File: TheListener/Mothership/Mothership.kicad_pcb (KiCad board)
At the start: 2 copper layers, 82 x 93.5 mm, 64 parts, among them J1 RJ45, J10 Conn_01x10_Female, J11 Conn_01x10_Female, J2 RJ45, J3 RJ45, J4 RJ45, J5 RJ45, J6 RJ45, J7 RJ45, J8 RJ45, U1 SP3491, U10 AMS1117-3.3, U2 SP3491, U3 SP3491, U4 SP3491, U5 SP3491, U6 SP3491, U7 SP3491, U8 SP3491, U9 AMS1117-3.3

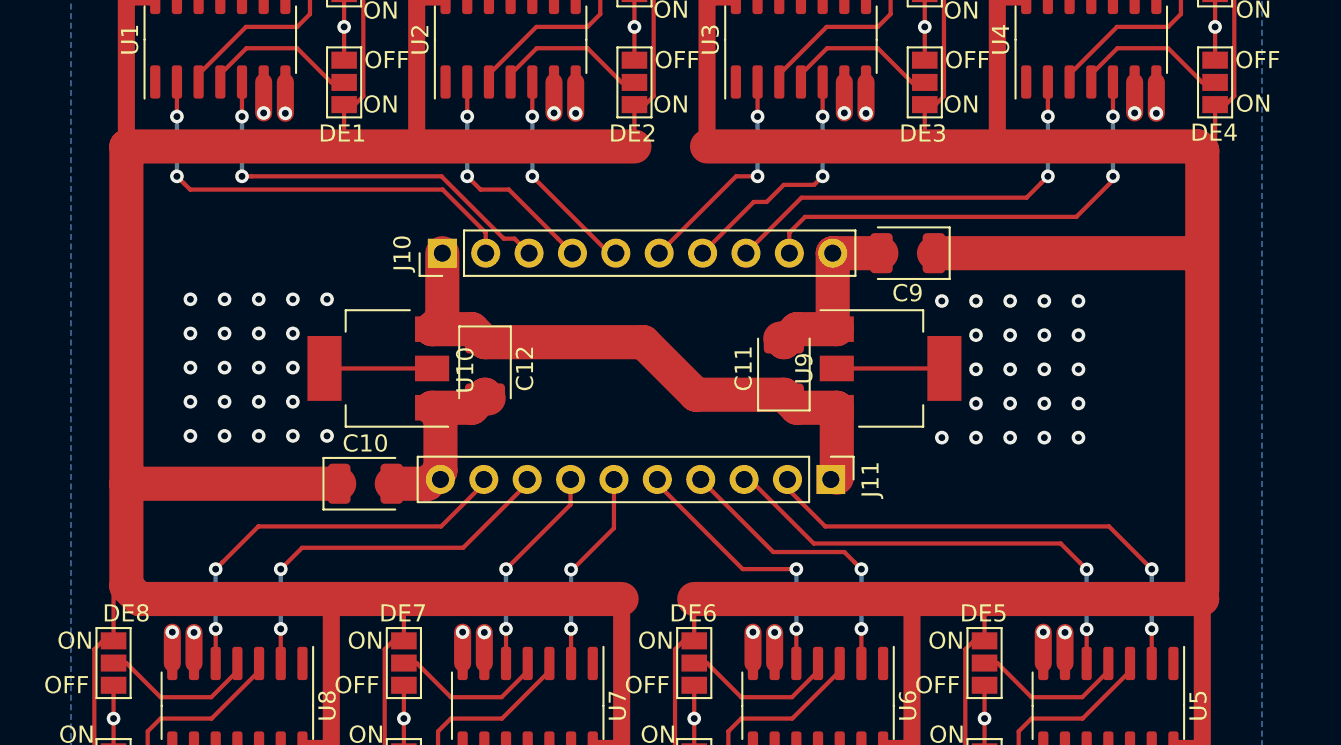
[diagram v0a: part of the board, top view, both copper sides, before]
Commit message: updates
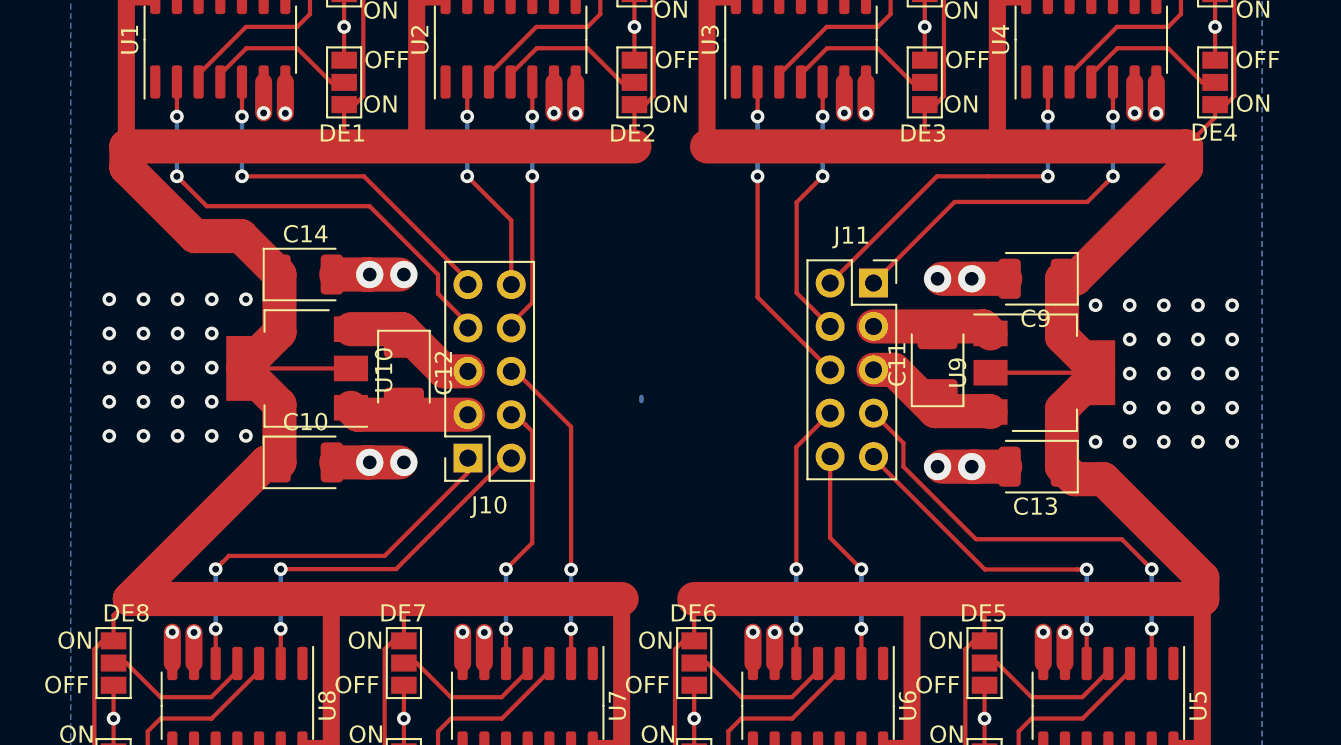
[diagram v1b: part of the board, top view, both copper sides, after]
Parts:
- added C13: 10uF, Capacitor_Tantalum_SMD:CP_EIA-3528-21_Kemet-B, F.Cu at (120.5, 73.8)
- added C14: 10uF, Capacitor_Tantalum_SMD:CP_EIA-3528-21_Kemet-B, F.Cu at (77.8, 62.5)
- C10, C9: value 22uF -> 10uF
- J10, J11: value Conn_01x10_Female -> Conn_02x05_Odd_Even; footprint Connector_PinHeader_2.54mm:PinHeader_1x10_P2.54mm_Vertical -> Connector_PinSocket_2.54mm:PinSocket_2x05_P2.54mm_Vertical
- moved J10 12.1 mm to (87.2, 73.2), turned to 180 degrees
- moved J11 11.8 mm to (111.0, 63.0), turned to 0 degrees
- moved C11 9.00 mm to (114.8, 67.8)
- moved U9 9.00 mm to (121.0, 68.2)
- moved C9 7.65 mm to (120.5, 62.8)
- moved C12 4.76 mm to (83.5, 68.2)
- moved U10 4.75 mm to (77.2, 68.0)
- moved C10 3.72 mm to (77.8, 73.5)
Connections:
- J10 pad 1: +5V -> T_5
- J10 pad 10: GND -> R_3
- J10 pad 2: R_4 -> R_5
- J10 pad 3: T_4 -> GND
- J10 pad 4: R_3 -> T_6
- J10 pad 5: T_3 -> +5V
- J10 pad 6: R_2 -> R_6
- J10 pad 7: T_2 -> R_4
- J10 pad 8: R_1 -> T_3
- J10 pad 9: T_1 -> T_4
- J11 pad 1: +5V -> T_1
- J11 pad 10: GND -> R_7
- J11 pad 2: R_8 -> R_1
- J11 pad 3: T_8 -> GND
- J11 pad 4: R_7 -> T_2
- J11 pad 5: T_7 -> +5V
- J11 pad 6: R_6 -> R_2
- J11 pad 7: T_6 -> R_8
- J11 pad 8: R_5 -> T_7
- J11 pad 9: T_5 -> T_8
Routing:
- net +5V: track 34.5 -> 15.7 mm
- net VCC1: track 205.7 -> 193.6 mm
- net GND: track 110.7 -> 118.9 mm, vias 92 -> 100
- net R_6: track 11.5 -> 18.8 mm
- net T_8: track 27.8 -> 20.7 mm
- net R_2: track 13.1 -> 18.6 mm
- net T_1: track 26.9 -> 21.5 mm
- net R_7: track 17.1 -> 12.9 mm
- net R_1: track 25.1 -> 20.9 mm
- net T_6: track 12.1 -> 16.0 mm
- net T_4: track 24.2 -> 21.3 mm
- net VCC2: track 199.4 -> 196.8 mm
- net R_8: track 28.8 -> 26.4 mm
- net T_3: track 12.3 -> 14.7 mm
- net T_2: track 14.4 -> 15.8 mm
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
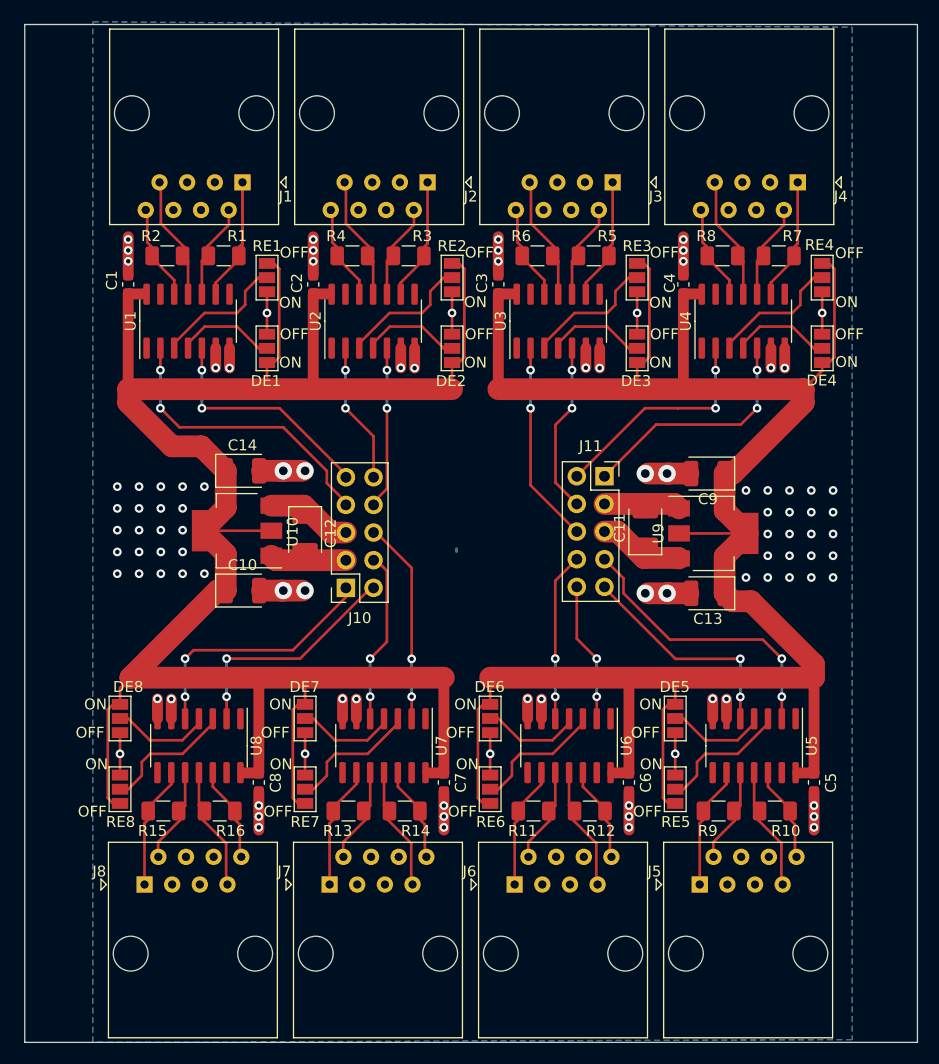
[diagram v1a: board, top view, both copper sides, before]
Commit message: final
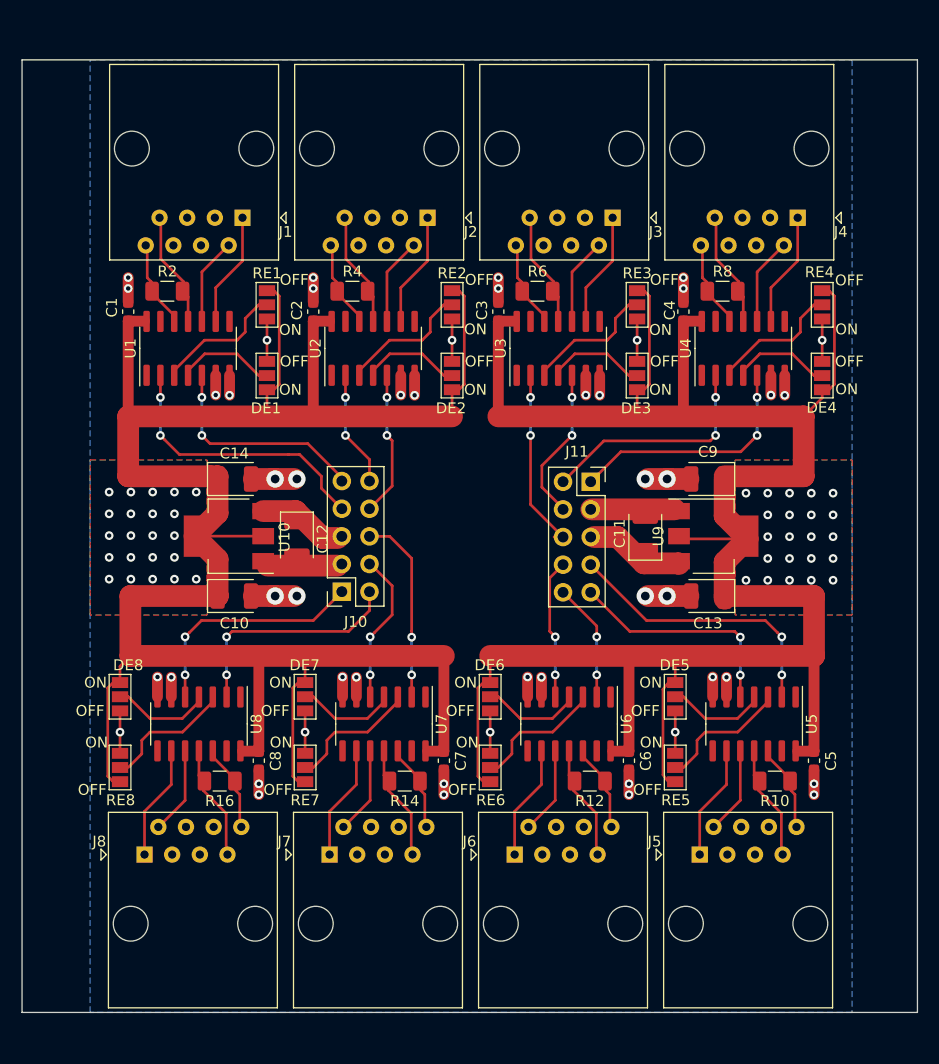
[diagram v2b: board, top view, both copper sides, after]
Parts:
- removed R1, R11, R13, R15, R3, R5, R7, R9: 100, Resistor_SMD:R_1206_3216Metric
- moved J1 3.25 mm to (77.8, 39.2)
- moved J2 3.25 mm to (94.8, 39.2)
- moved J3 3.25 mm to (111.8, 39.2)
- moved J4 3.25 mm to (128.8, 39.2)
- moved R2 3.25 mm to (70.8, 46.0)
- moved R4 3.25 mm to (87.8, 46.0)
- moved R6 3.25 mm to (104.8, 46.0)
- moved R8 3.25 mm to (121.8, 46.0)
- moved J5 2.75 mm to (119.8, 97.8)
- moved J6 2.75 mm to (102.8, 97.8)
- moved J7 2.75 mm to (85.8, 97.8)
- moved J8 2.75 mm to (68.8, 97.8)
- moved R10 2.75 mm to (126.7, 91.0)
- moved R12 2.75 mm to (109.7, 91.0)
- moved R14 2.75 mm to (92.7, 91.0)
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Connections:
- C11 pad 1: +5V -> 5VDC_1
- C12 pad 1: +5V -> 5VDC_2
- J10 pad 5: +5V -> 5VDC_2
- J11 pad 5: +5V -> 5VDC_1
- U10 pad 3: +5V -> 5VDC_2
- U9 pad 3: +5V -> 5VDC_1
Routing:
- net +5V: track 15.7 -> 0.00 mm
- net VCC2: track 196.8 -> 207.2 mm, vias 0 -> 22
- net GND: track 118.9 -> 108.7 mm, vias 100 -> 48
- net VCC1: track 193.6 -> 203.1 mm, vias 0 -> 22
- net 5VDC_1: track 0.00 -> 8.83 mm
- net 5VDC_2: track 0.00 -> 7.87 mm
- net Net-(J1-Pad1): track 17.4 -> 11.3 mm
- net T_7: track 15.5 -> 12.9 mm
- net T_5: track 23.7 -> 21.6 mm
- net T_6: track 16.0 -> 13.9 mm
- net R_3: track 12.7 -> 10.6 mm
- net R_7: track 12.9 -> 10.9 mm
- net T_2: track 15.8 -> 14.3 mm
- net R_6: track 18.8 -> 17.4 mm
- net T_3: track 14.7 -> 13.3 mm
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- added copper zone on B.Cu, net VCC1
- added copper zone on F.Cu, net VCC1
- added copper zone on B.Cu, net VCC2
- added copper zone on F.Cu, net VCC2
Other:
- board size 82 x 93.5 mm -> 82.2 x 87.5 mm

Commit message: working
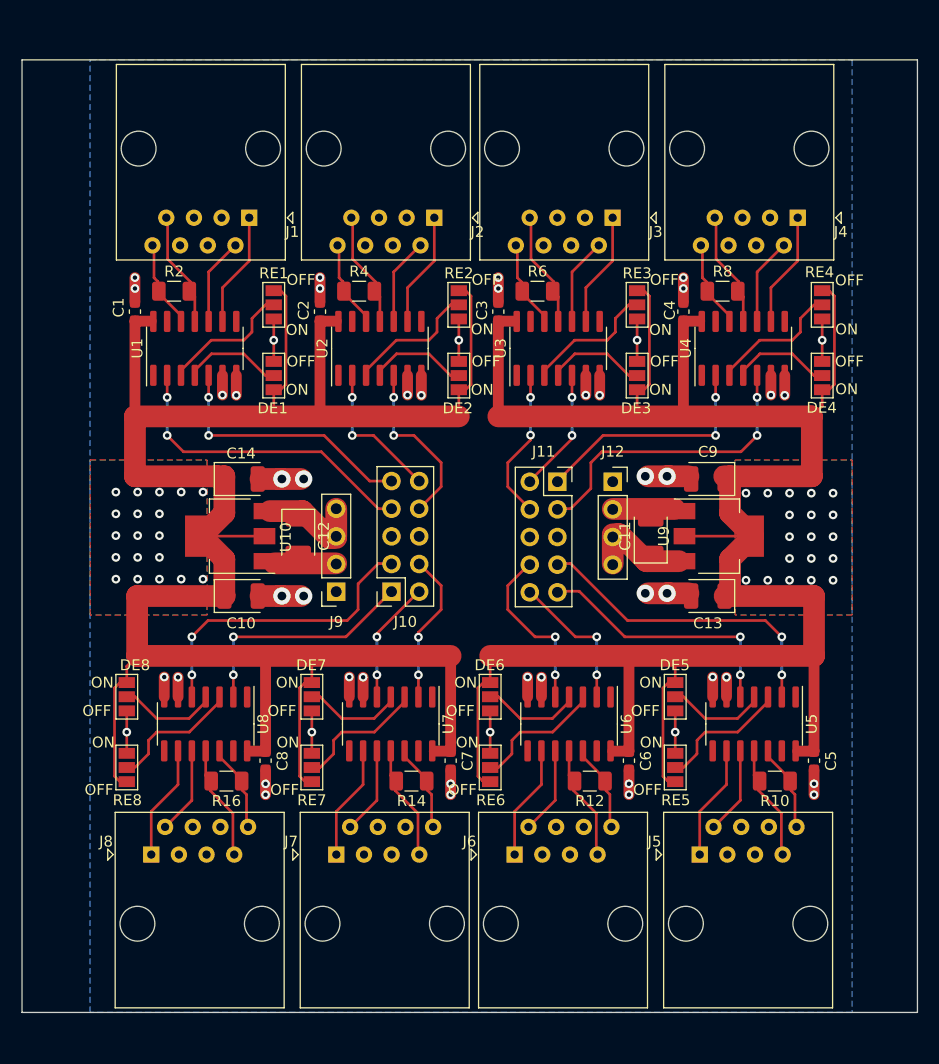
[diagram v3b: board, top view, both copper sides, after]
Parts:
- added J12: Conn_01x04_Male, Connector_PinSocket_2.54mm:PinSocket_1x04_P2.54mm_Vertical, F.Cu at (111.8, 63.5)
- added J9: Conn_01x04_Male, Connector_PinSocket_2.54mm:PinSocket_1x04_P2.54mm_Vertical, F.Cu at (86.4, 73.6)
- moved J10 4.56 mm to (91.4, 73.6)
- moved J11 3.05 mm to (106.7, 63.5)
- moved C1 0.62 mm to (67.9, 47.9)
- moved C10 0.62 mm to (77.6, 74.0)
- moved C14 0.62 mm to (77.6, 63.2)
- moved C2 0.62 mm to (84.9, 47.9)
- moved C7 0.62 mm to (96.9, 89.1)
- moved C8 0.62 mm to (79.9, 89.1)
- moved DE1 0.62 mm to (80.6, 53.8)
- moved DE2 0.62 mm to (97.6, 53.8)
- moved DE7 0.62 mm to (84.1, 83.2)
- moved DE8 0.62 mm to (67.1, 83.2)
- moved J1 0.62 mm to (78.4, 39.2)
- moved J2 0.62 mm to (95.4, 39.2)
- moved J7 0.62 mm to (86.4, 97.8)
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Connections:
- J10 pad 1: T_5 -> R_5
- J10 pad 2: R_5 -> T_6
- J10 pad 3: GND -> T_5
- J10 pad 4: T_6 -> R_6
- J10 pad 5: 5VDC_2 -> (no net)
- J10 pad 6: R_6 -> (no net)
- J11 pad 1: T_1 -> R_1
- J11 pad 2: R_1 -> T_2
- J11 pad 3: GND -> T_1
- J11 pad 4: T_2 -> R_2
- J11 pad 5: 5VDC_1 -> (no net)
- J11 pad 6: R_2 -> (no net)
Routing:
- net T_5: track 21.6 -> 28.0 mm
- net T_1: track 22.6 -> 28.0 mm
- net VCC1: track 203.1 -> 207.2 mm, vias 22 -> 19
- net T_4: track 20.2 -> 24.1 mm
- net R_6: track 17.4 -> 14.0 mm
- net R_2: track 17.3 -> 14.0 mm
- net R_4: track 25.6 -> 28.9 mm
- net T_7: track 12.9 -> 16.0 mm
- net R_8: track 25.8 -> 28.9 mm
- net T_8: track 21.0 -> 24.1 mm
- net T_2: track 14.3 -> 11.4 mm
- net R_3: track 10.6 -> 13.4 mm
- net GND: track 108.7 -> 106.0 mm
- net T_3: track 13.3 -> 16.0 mm
- net T_6: track 13.9 -> 11.4 mm
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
